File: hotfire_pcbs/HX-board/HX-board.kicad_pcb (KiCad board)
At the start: 2 copper layers, 101.5 x 88.5 mm, 54 parts, among them J1 Testpoints, J2 PCIE-LP-01-01-F-DV-A-TR, J3 DB15_Female, J4 Testpoints, J5 DB15_Female, J6 Testpoints, U1 HX711_Breakout, U2 HX711_Breakout, U3 HX711_Breakout, U4 HX711_Breakout, U5 HX711_Breakout

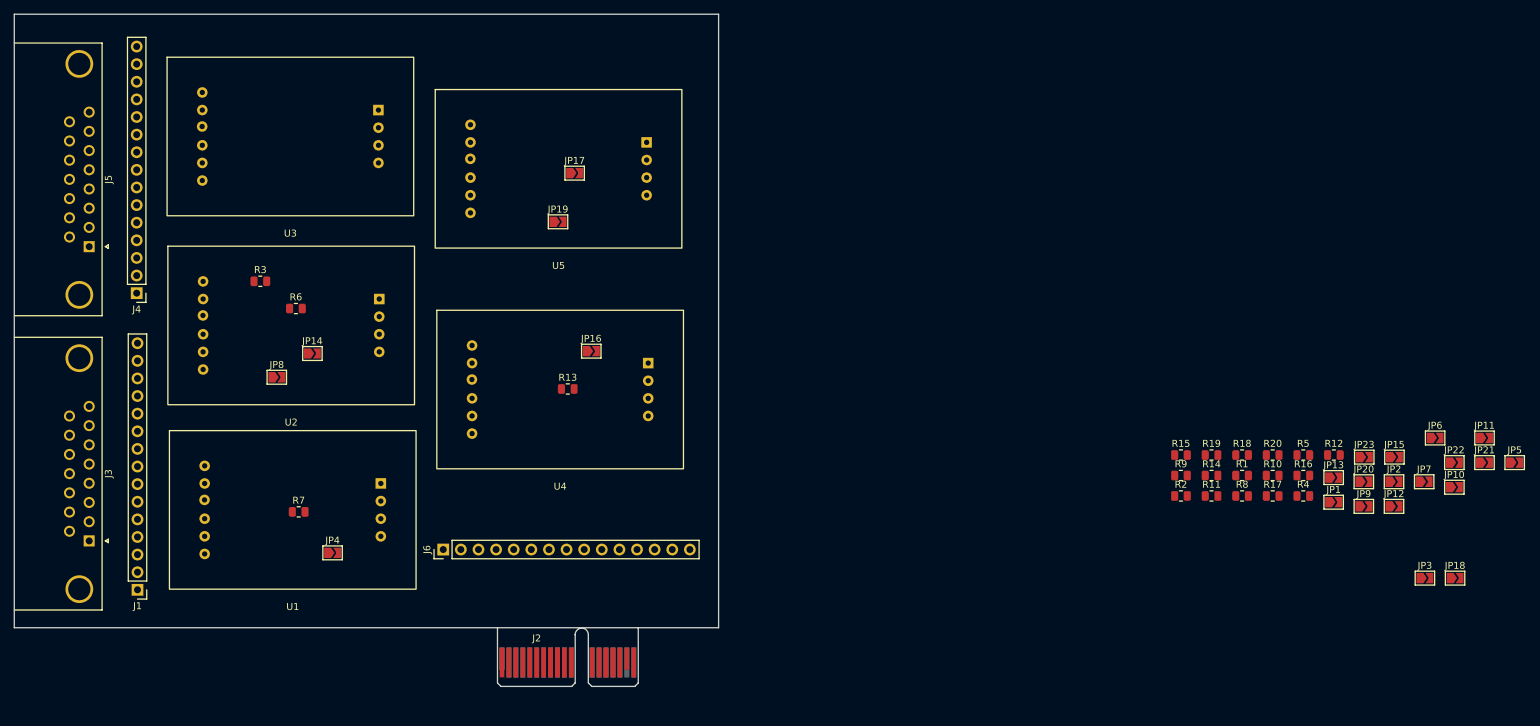
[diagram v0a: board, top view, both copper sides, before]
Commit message: Updated HX711 Board
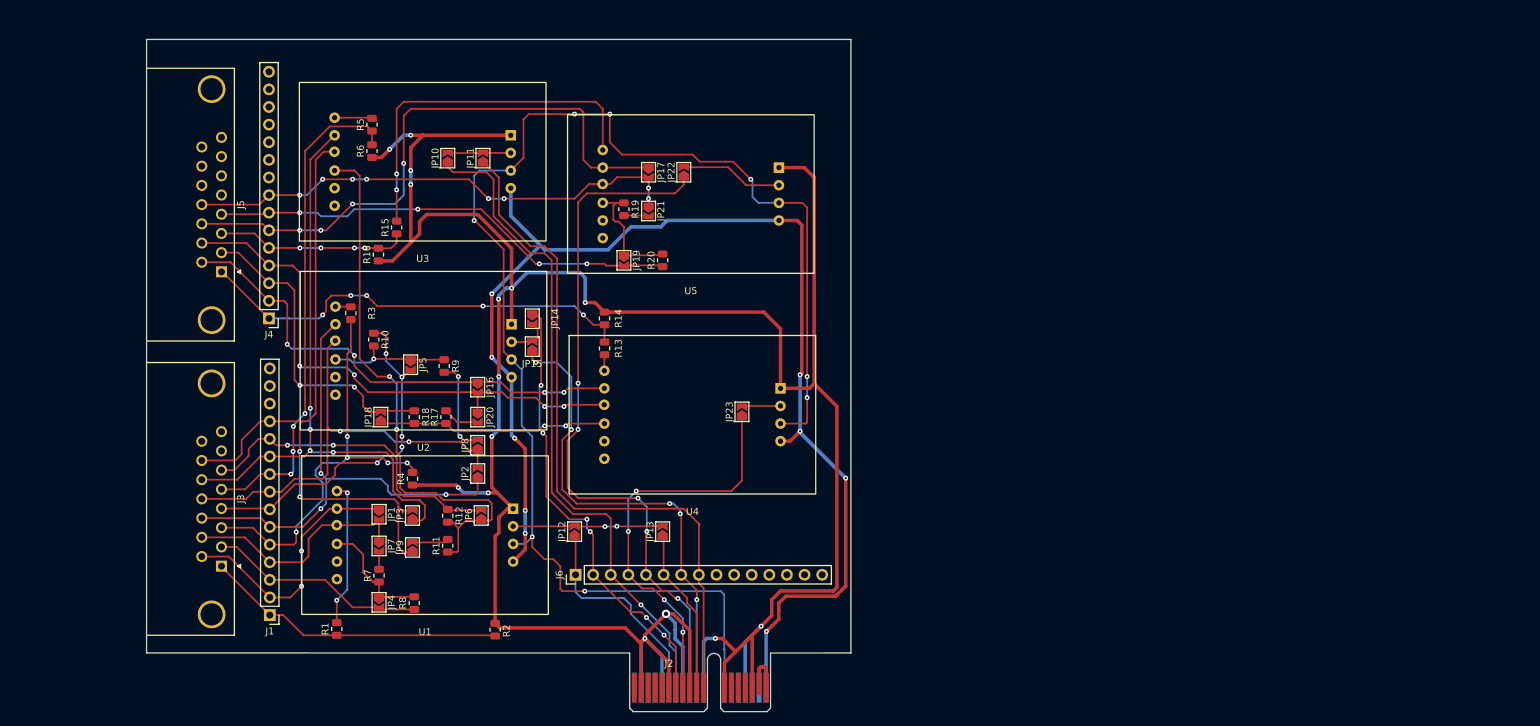
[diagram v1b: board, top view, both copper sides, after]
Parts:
- J6: value Testpoints -> PCIe_1
- moved JP5 159.8 mm to (148.8, 80.9), turned to -90 degrees
- moved JP18 156.6 mm to (144.6, 88.5), turned to 90 degrees
- moved JP10 152.7 mm to (154.2, 51.1), turned to 90 degrees
- moved JP7 151.0 mm to (144.3, 107.1), turned to -90 degrees
- moved JP11 149.9 mm to (159.3, 51.1), turned to 90 degrees
- moved JP3 146.3 mm to (149.1, 102.7), turned to 90 degrees
- moved R5 142.5 mm to (143.3, 46.3), turned to 90 degrees
- moved JP6 138.0 mm to (159.0, 102.7), turned to 90 degrees
- moved JP1 137.7 mm to (144.3, 102.5), turned to -90 degrees
- moved JP9 137.3 mm to (149.1, 107.3), turned to 90 degrees
- moved R16 137.1 mm to (144.2, 65.0), turned to 90 degrees
- moved R1 132.4 mm to (138.2, 119.0), turned to 90 degrees
- moved JP2 132.1 mm to (158.5, 96.6), turned to 90 degrees
- moved R10 131.1 mm to (143.5, 77.3), turned to -90 degrees
- moved R4 128.5 mm to (149.1, 97.4), turned to 90 degrees
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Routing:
- net GND: track 0.00 -> 402.0 mm, vias 0 -> 15
- net /HX_CLK: track 0.00 -> 205.3 mm, vias 0 -> 8
- net +5V: track 0.00 -> 187.1 mm, vias 0 -> 9
- net /PCIe_5: track 0.00 -> 101.2 mm, vias 0 -> 5
- net /PCIe_8: track 0.00 -> 99.4 mm
- net /PT3_A-: track 0.00 -> 96.8 mm, vias 0 -> 2
- net /PCIe_3: track 0.00 -> 96.1 mm, vias 0 -> 1
- net /PT3_E-: track 0.00 -> 90.5 mm, vias 0 -> 4
- net /PT5_E-: track 0.00 -> 86.3 mm, vias 0 -> 4
- net Net-(JP6-Pad1): track 0.00 -> 80.9 mm, vias 0 -> 2
- net /PT4_A-: track 0.00 -> 78.9 mm, vias 0 -> 4
- net /PT5_A-: track 0.00 -> 72.5 mm, vias 0 -> 8
- net /PT2_E-: track 0.00 -> 72.3 mm, vias 0 -> 3
- net /PT3_E+: track 0.00 -> 71.8 mm, vias 0 -> 4
- net /PT4_E-: track 0.00 -> 70.3 mm, vias 0 -> 4
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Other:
- board size 101.5 x 88.5 mm -> 101.6 x 88.5 mm
